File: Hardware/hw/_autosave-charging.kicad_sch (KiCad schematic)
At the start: 7 parts, among them J1 Screw_Terminal_01x02, J2 Screw_Terminal_01x02, Q2 PMOS, Q3 PMOS, U3 INA219, U7 BQ24650

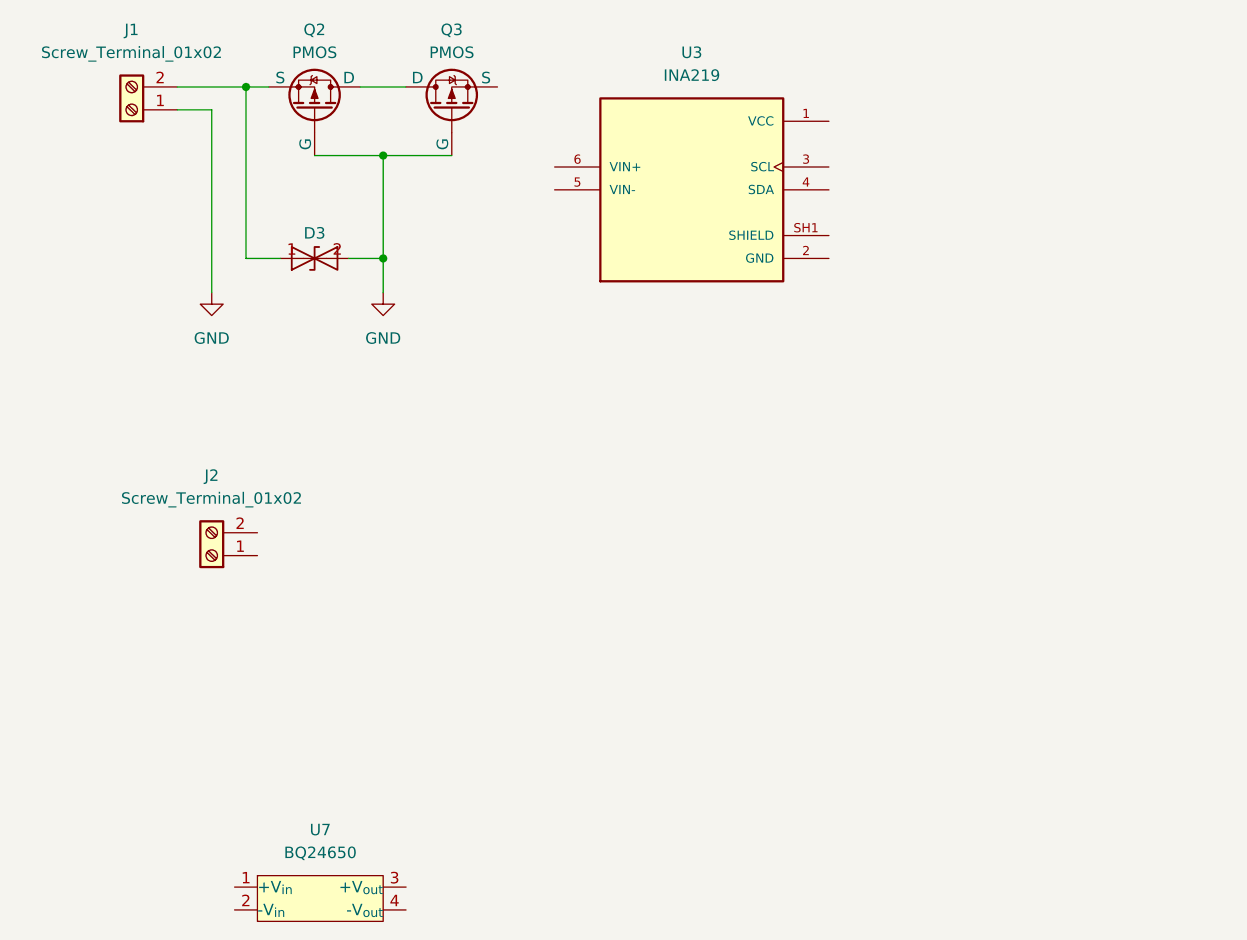
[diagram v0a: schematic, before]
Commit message: HW update
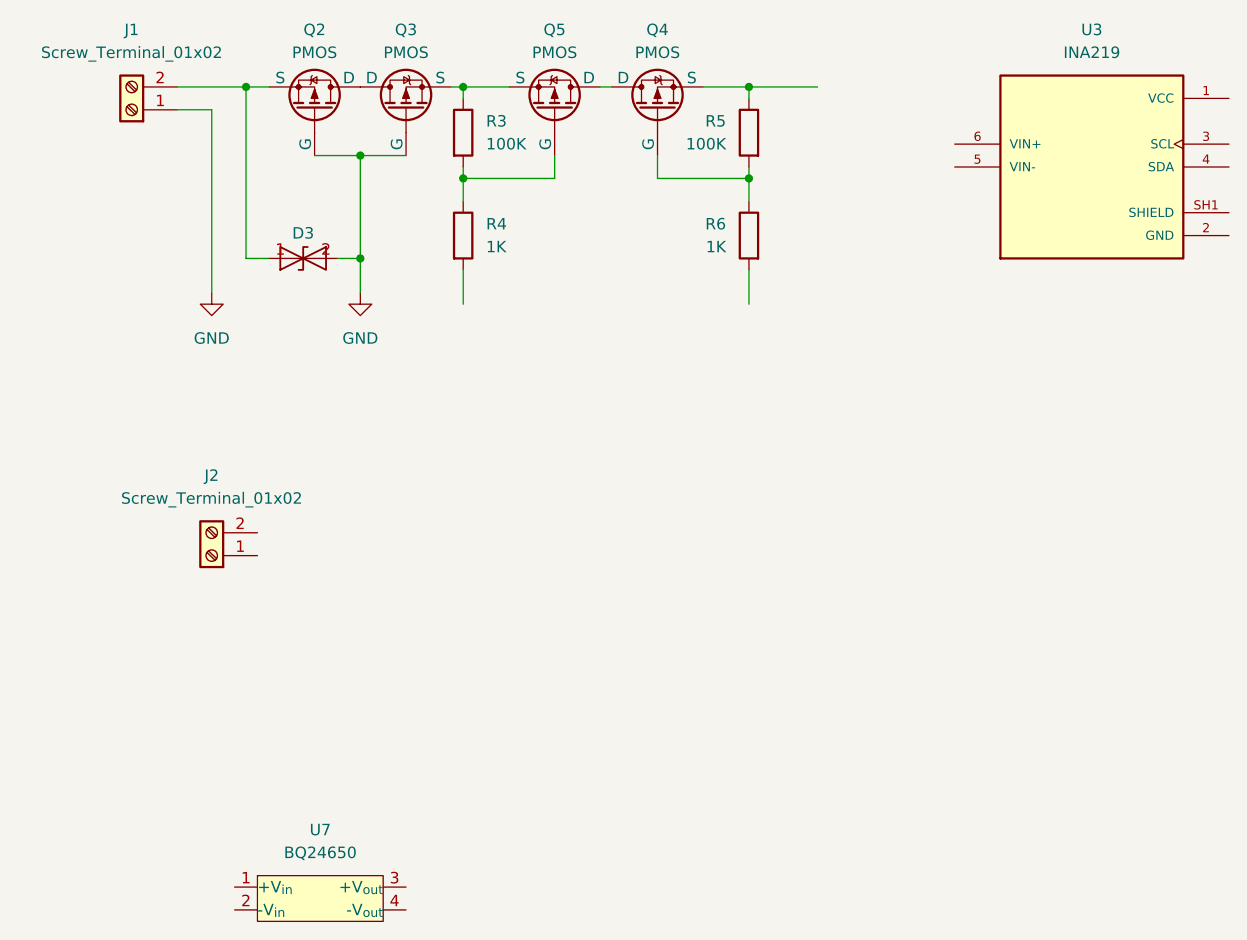
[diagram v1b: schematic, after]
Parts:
- added Q4, Q5: PMOS, symbol Simulation_SPICE:PMOS
- added R3, R5: 100K, symbol Device:R
- added R4, R6: 1K, symbol Device:R
- D3: footprint (none) -> SMBJ24CA:DO214AA
- U3: footprint INA219:MODULE_INA219 -> INA219_Module:MODULE_INA219
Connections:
- net at Q3.3 (S): now also Q5.3 (S), R3.1
- new net: Q4.1 (D), Q5.1 (D)
- new net: Q4.2 (G), R5.2, R6.1
- new net: Q4.3 (S), R5.1
- new net: Q5.2 (G), R3.2, R4.1
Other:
- moved on the sheet: D3, Q3
